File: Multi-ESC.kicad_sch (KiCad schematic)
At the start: 1 part, among them U3 LMR51450FN

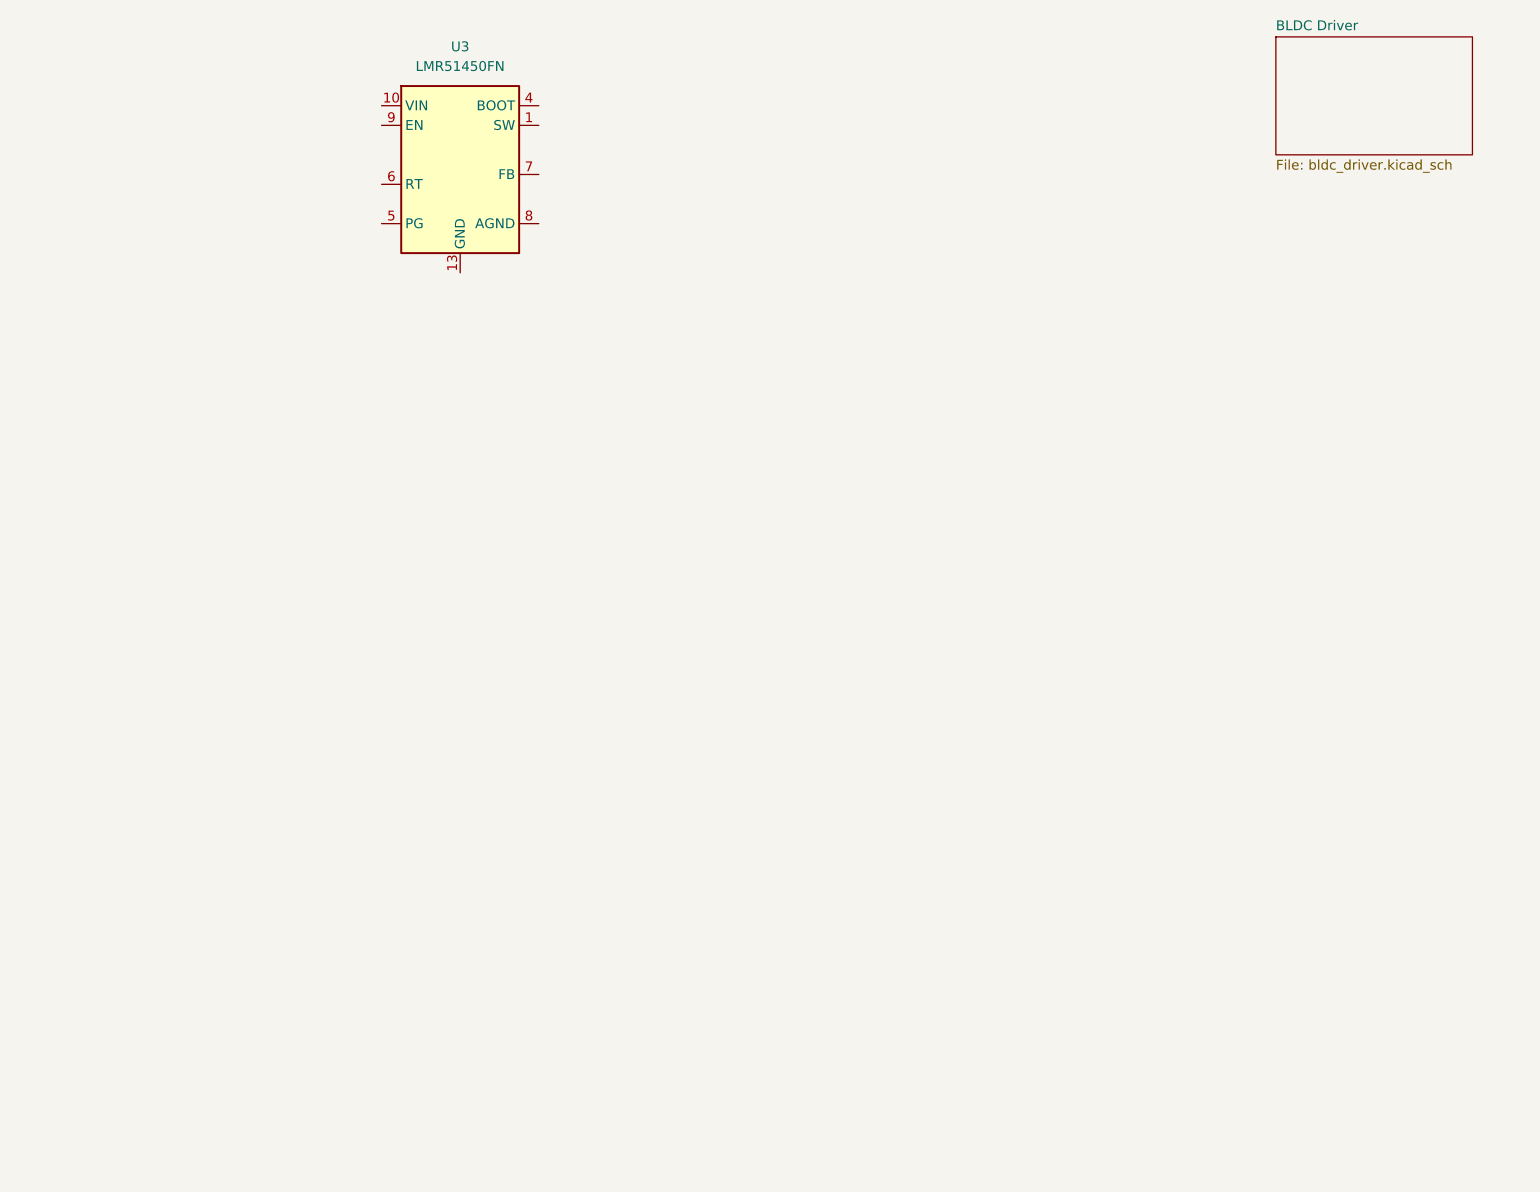
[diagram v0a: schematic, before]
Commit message: wired regulator
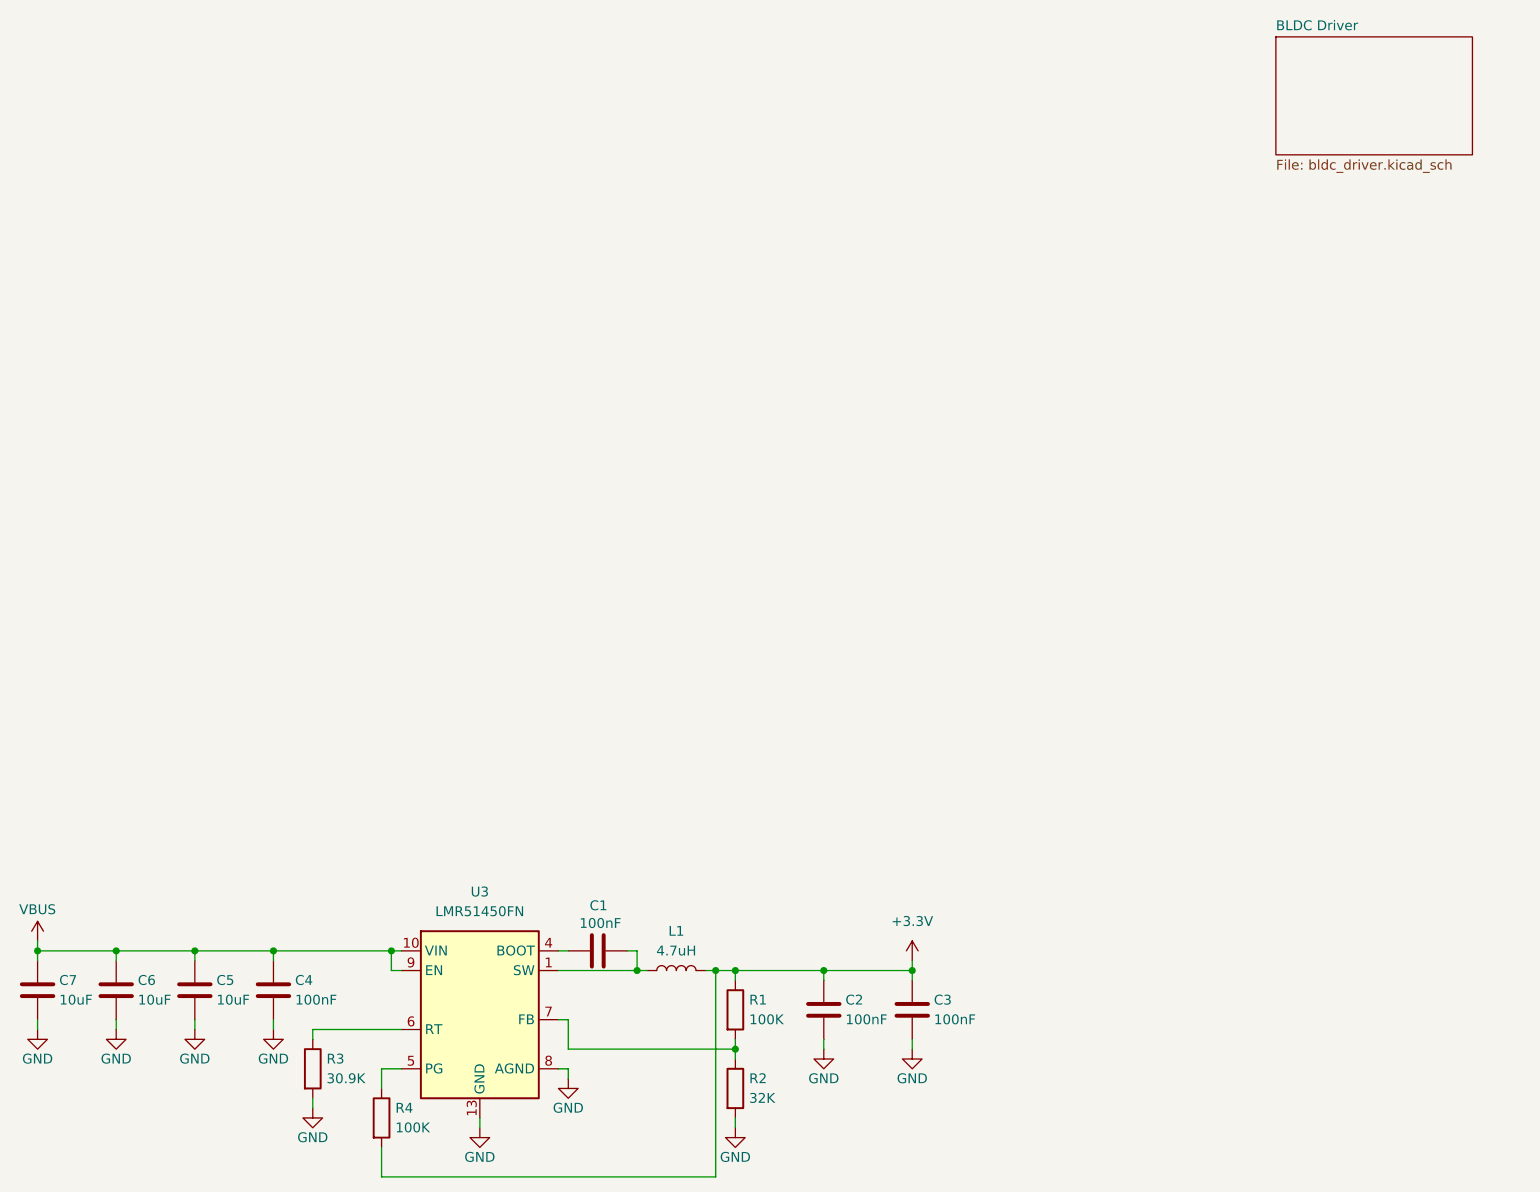
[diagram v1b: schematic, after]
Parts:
- added C1, C2, C3, C4: 100nF, symbol Device:C
- added C5, C6, C7: 10uF, symbol Device:C
- added L1: 4.7uH, symbol Device:L
- added R1, R4: 100K, symbol Device:R
- added R2: 32K, symbol Device:R
- added R3: 30.9K, symbol Device:R
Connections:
- net VIN is gone; now on net VBUS: U3.10 (VIN), U3.11 (VIN), U3.12 (VIN)
- net at U3.1 (SW), U3.2 (SW), U3.3 (SW): now also C1.2, L1.1
- net GND: now reaches U3.13 (GND)
- net GND: now also U3.8 (AGND), C2.2, C3.2, C4.2, C5.2, C6.2, C7.2, R2.2, R3.2
- net at U3.4 (BOOT): now also C1.1
- net at U3.5 (PG): now also R4.1
- net at U3.6 (RT): now also R3.1
- net at U3.7 (FB): now also R1.2, R2.1
- net VBUS: now reaches U3.9 (EN)
- net VBUS: now also C4.1, C5.1, C6.1, C7.1
- new net +3.3V: C2.1, C3.1, L1.2, R1.1, R4.2
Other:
- moved on the sheet: U3
